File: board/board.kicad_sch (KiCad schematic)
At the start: 4 parts, among them J1 Conn_01x02_Pin, J2 Conn_01x02_Pin, J3 003_power

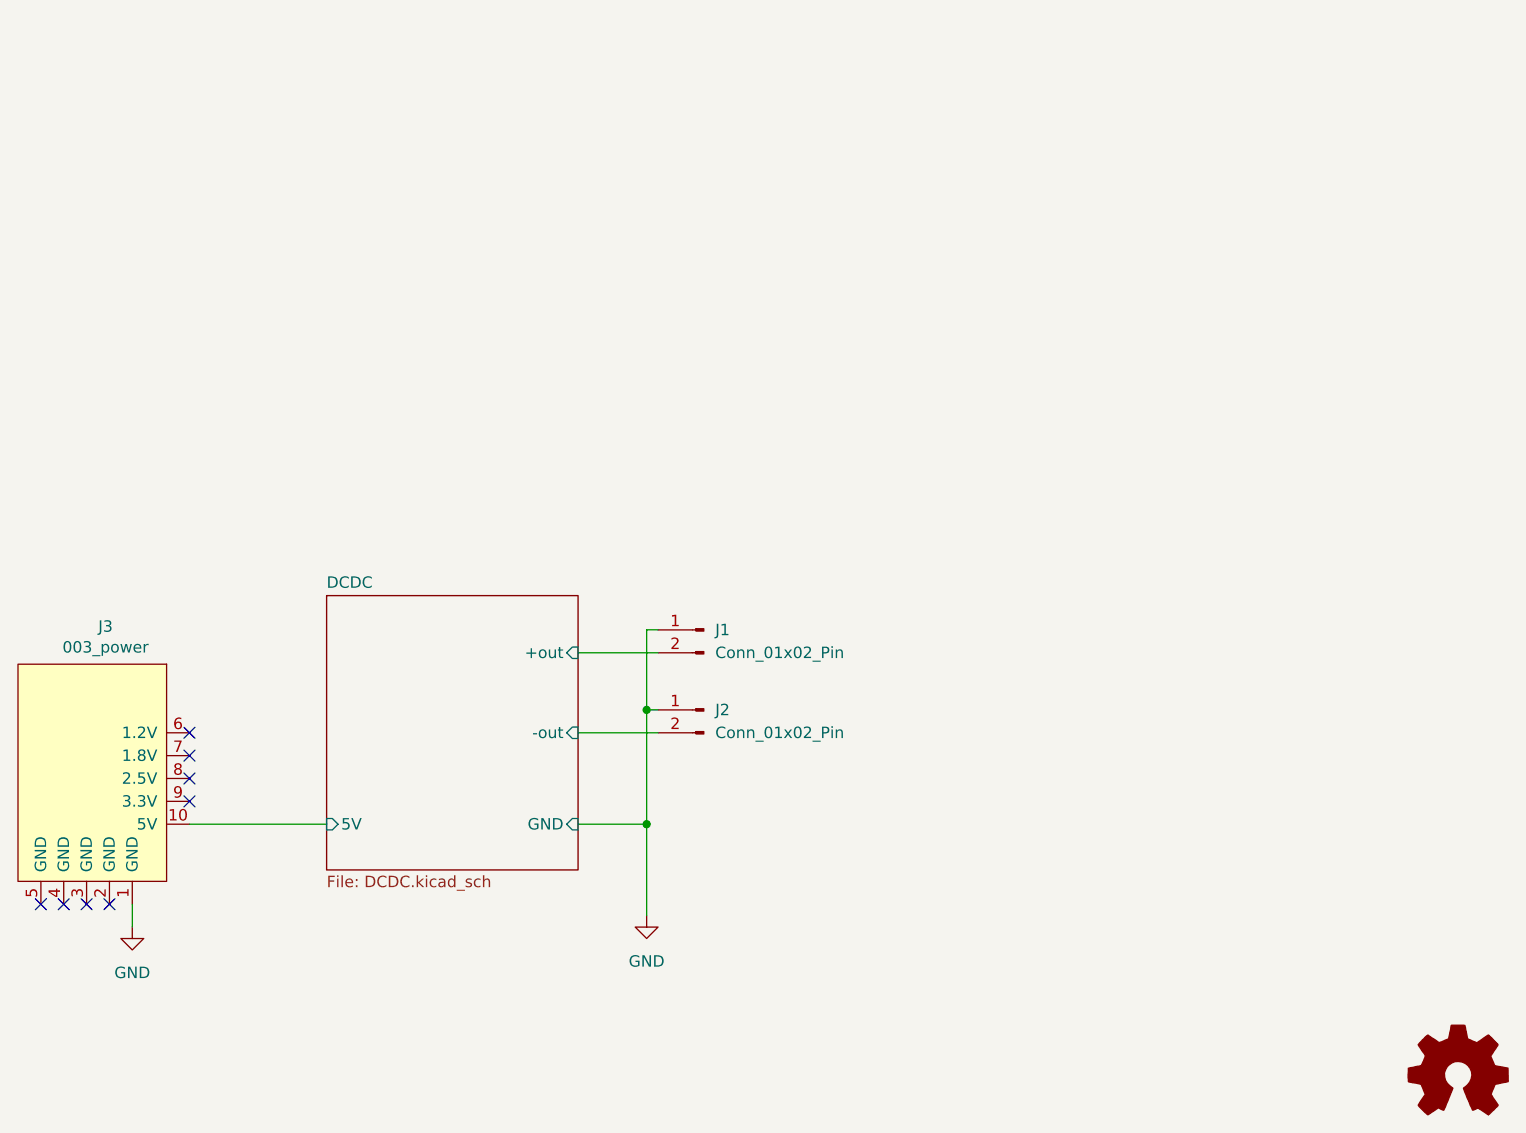
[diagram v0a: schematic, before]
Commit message: initial b147
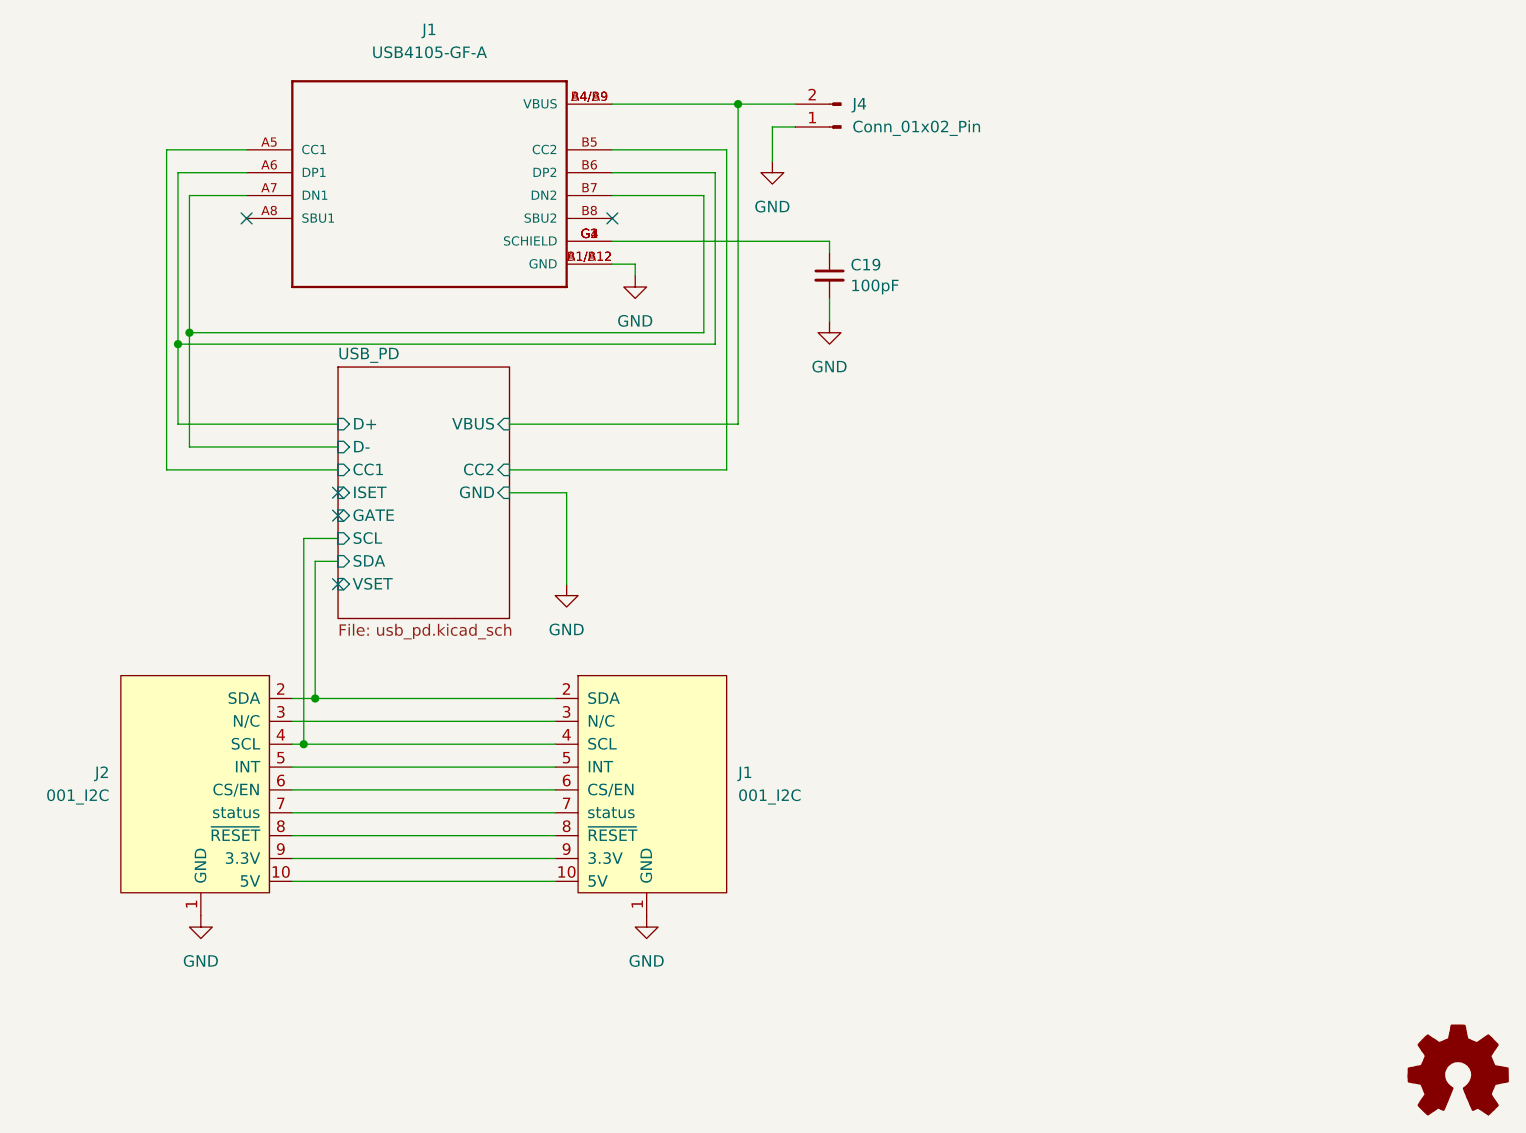
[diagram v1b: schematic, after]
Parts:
- removed J1, J2: Conn_01x02_Pin, Connector_PinHeader_2.54mm:PinHeader_1x02_P2.54mm_Vertical, symbol Connector:Conn_01x02_Pin
- removed J3: 003_power, on_edge:on_edge_2x05_device, symbol put_on_edge:003_power
- added C19: 100pF, Capacitor_SMD:C_0402_1005Metric, symbol Device:C_Small
- added J1: USB4105-GF-A, b051:GCT_USB4105-GF-A, symbol b051:USB4105-GF-A
- added J1: 001_I2C, on_edge:on_edge_2x05_host, symbol put_on_edge:001_I2C
- added J2: 001_I2C, on_edge:on_edge_2x05_device, symbol put_on_edge:001_I2C
- added J4: Conn_01x02_Pin, Connector_PinHeader_2.54mm:PinHeader_1x02_P2.54mm_Vertical, symbol Connector:Conn_01x02_Pin
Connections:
- net GND: now also C19.2, J1.1 (GND), J1.A1/B12 (GND), J1.B1/A12 (GND), J2.1 (GND), J4.1 (Pin_1)
- new net: C19.1, J1.G1 (SCHIELD), J1.G2 (SCHIELD), J1.G3 (SCHIELD), J1.G4 (SCHIELD)
- new net: J1.10 (5V), J2.10 (5V)
- new net: J1.3 (N/C), J2.3 (N/C)
- new net: J1.5 (INT), J2.5 (INT)
- new net: J1.6 (CS/EN), J2.6 (CS/EN)
- new net: J1.7 (status), J2.7 (status)
- new net: J1.8 (~{RESET}), J2.8 (~{RESET})
- new net: J1.9 (3.3V), J2.9 (3.3V)
- new net USB_PD/CC1: J1.A5 (CC1)
- new net USB_PD/CC2: J1.B5 (CC2)
- new net USB_PD/D+: J1.A6 (DP1), J1.B6 (DP2)
- new net USB_PD/D-: J1.A7 (DN1), J1.B7 (DN2)
- new net USB_PD/SCL: J1.4 (SCL), J2.4 (SCL)
- new net USB_PD/SDA: J1.2 (SDA), J2.2 (SDA)
- new net USB_PD/VBUS: J1.A4/B9 (VBUS), J1.B4/A9 (VBUS), J4.2 (Pin_2)
- no-connect marks 8 -> 5
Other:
- removed sheet DCDC
- added sheet USB_PD (usb_pd.kicad_sch)
